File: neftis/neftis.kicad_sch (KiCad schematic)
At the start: 32 parts, among them Q1 BC847, Q2 BC847, U1 ESP32-S3-WROOM-1, U2 QRE1113, U3 QRE1113, U7 QRE1113, U8 QRE1113

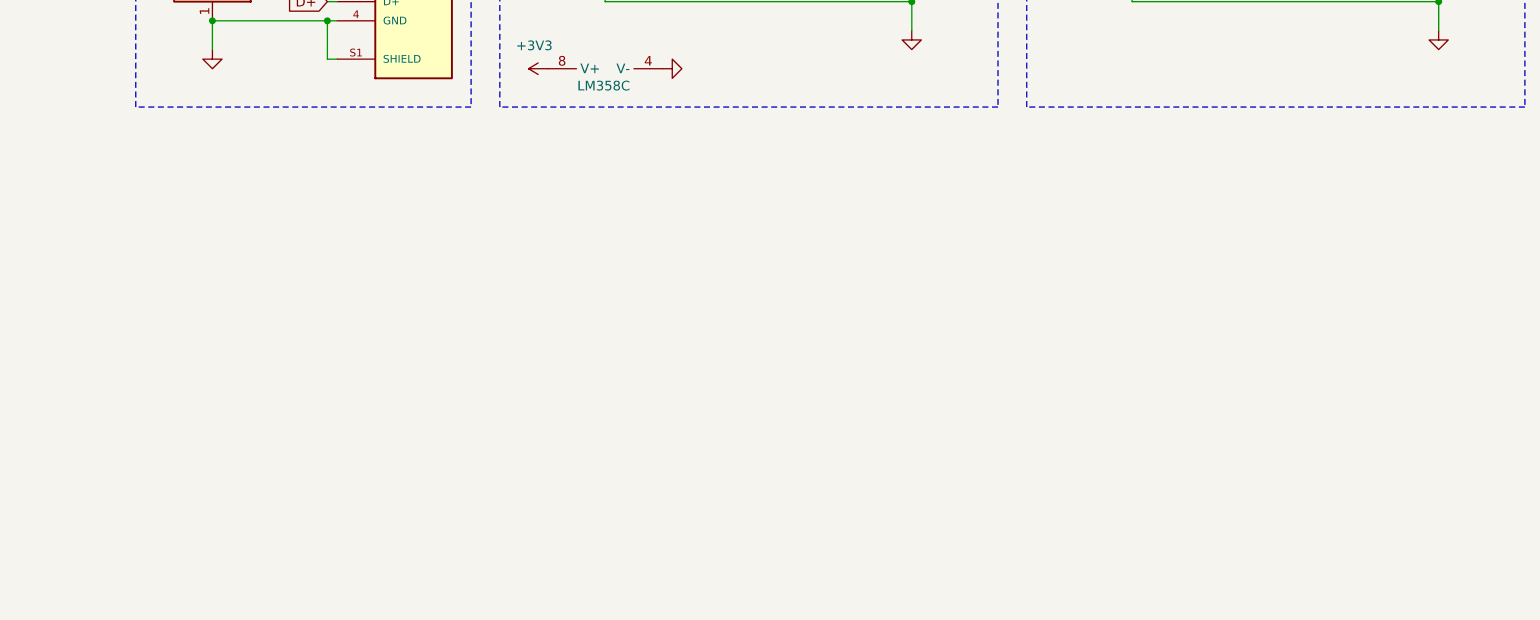
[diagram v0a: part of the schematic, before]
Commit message: ponte H
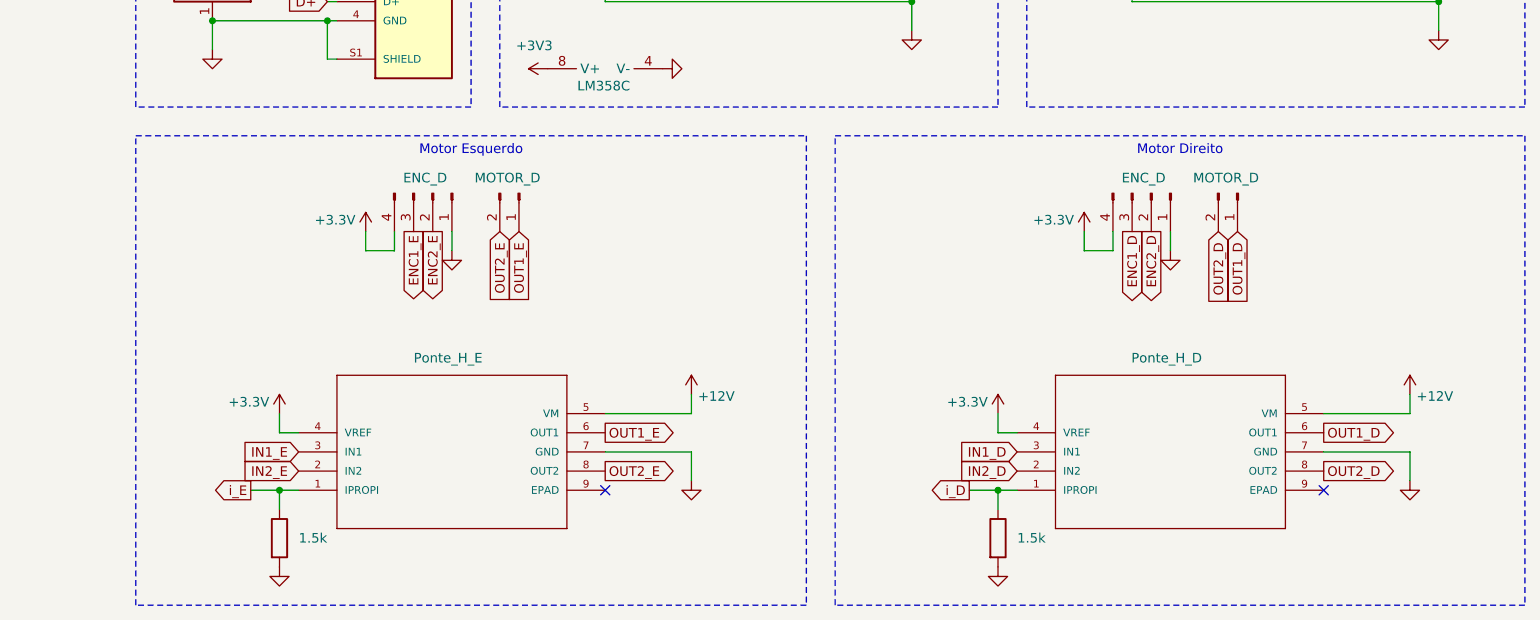
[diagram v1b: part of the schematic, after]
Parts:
- added Conn_01x02_Pin1, Conn_01x02_Pin3: MOTOR_D, Connector_PinSocket_2.54mm:PinSocket_1x02_P2.54mm_Vertical, symbol Connector:Conn_01x02_Pin
- added Conn_01x04_Pin1, Conn_01x04_Pin2: ENC_D, Connector_PinSocket_2.54mm:PinSocket_1x04_P2.54mm_Vertical, symbol Connector:Conn_01x04_Pin
- added DRV8251ADDAR1: Ponte_H_E, Library:ponte_H, symbol DRV8251ADDAR:DRV8251ADDAR
- added DRV8251ADDAR2: Ponte_H_D, Library:ponte_H, symbol DRV8251ADDAR:DRV8251ADDAR
- added R10, R11: 1.5k, Resistor_SMD:R_0805_2012Metric_Pad1.20x1.40mm_HandSolder, symbol Device:R
- renumbered Conn_01x02_Pin to Conn_01x02_Pin2, USB-B-S-X-X-TH to USB-B-S-X-X-TH1
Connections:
- net +3.3V: now also Conn_01x04_Pin1.4 (Pin_4), Conn_01x04_Pin2.4 (Pin_4), DRV8251ADDAR1.4 (VREF), DRV8251ADDAR2.4 (VREF)
- net GND: now also Conn_01x04_Pin1.1 (Pin_1), Conn_01x04_Pin2.1 (Pin_1), DRV8251ADDAR1.7 (GND), DRV8251ADDAR2.7 (GND), R10.2, R11.2
- new net +12V: DRV8251ADDAR1.5 (VM), DRV8251ADDAR2.5 (VM)
- new net ENC1_D: Conn_01x04_Pin2.3 (Pin_3)
- new net ENC1_E: Conn_01x04_Pin1.3 (Pin_3)
- new net ENC2_D: Conn_01x04_Pin2.2 (Pin_2)
- new net ENC2_E: Conn_01x04_Pin1.2 (Pin_2)
- new net IN1_D: DRV8251ADDAR2.3 (IN1)
- new net IN1_E: DRV8251ADDAR1.3 (IN1)
- new net IN2_D: DRV8251ADDAR2.2 (IN2)
- new net IN2_E: DRV8251ADDAR1.2 (IN2)
- new net OUT1_D: Conn_01x02_Pin3.1 (Pin_1), DRV8251ADDAR2.6 (OUT1)
- new net OUT1_E: Conn_01x02_Pin1.1 (Pin_1), DRV8251ADDAR1.6 (OUT1)
- new net OUT2_D: Conn_01x02_Pin3.2 (Pin_2), DRV8251ADDAR2.8 (OUT2)
- new net OUT2_E: Conn_01x02_Pin1.2 (Pin_2), DRV8251ADDAR1.8 (OUT2)
- new net i_D: DRV8251ADDAR2.1 (IPROPI), R10.1
- new net i_E: DRV8251ADDAR1.1 (IPROPI), R11.1
- no-connect marks 0 -> 2
